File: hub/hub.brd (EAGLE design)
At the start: 28.2 x 25.4 mm, 5 parts

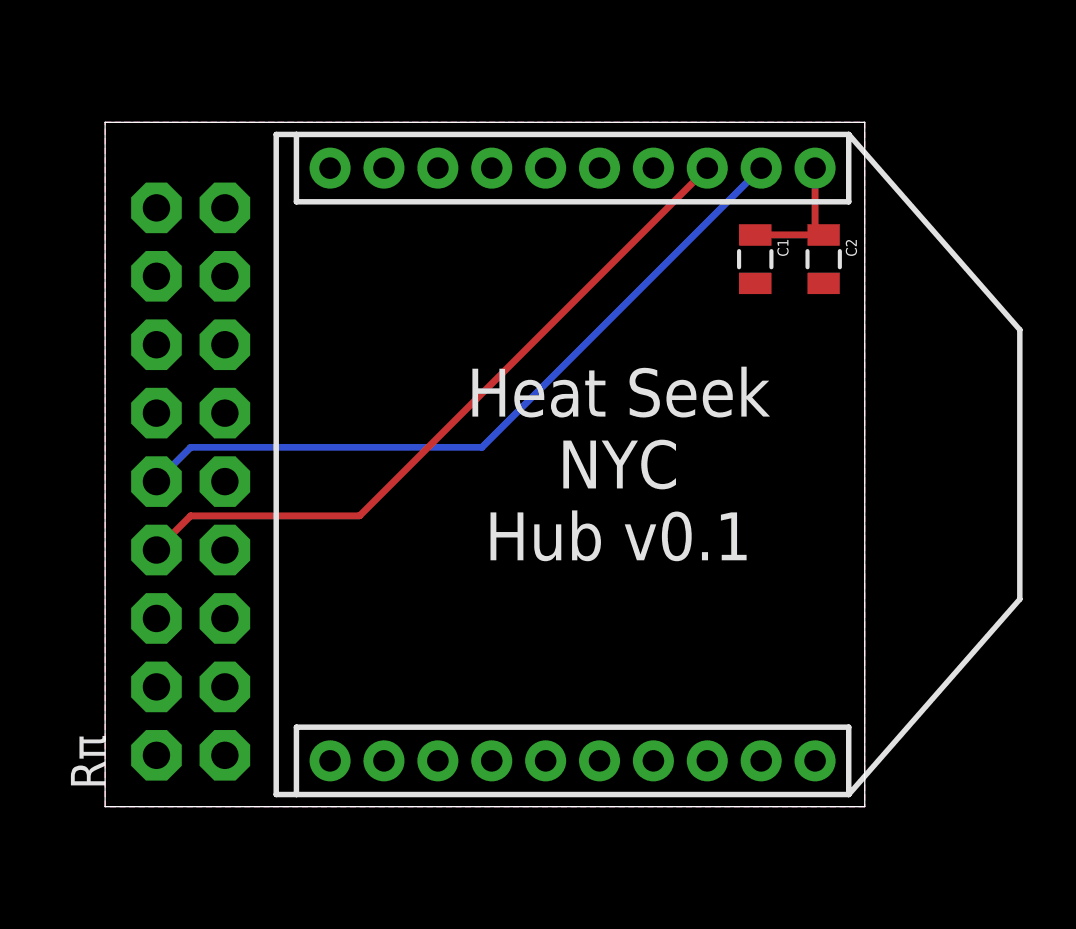
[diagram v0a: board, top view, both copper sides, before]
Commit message: smd-ver
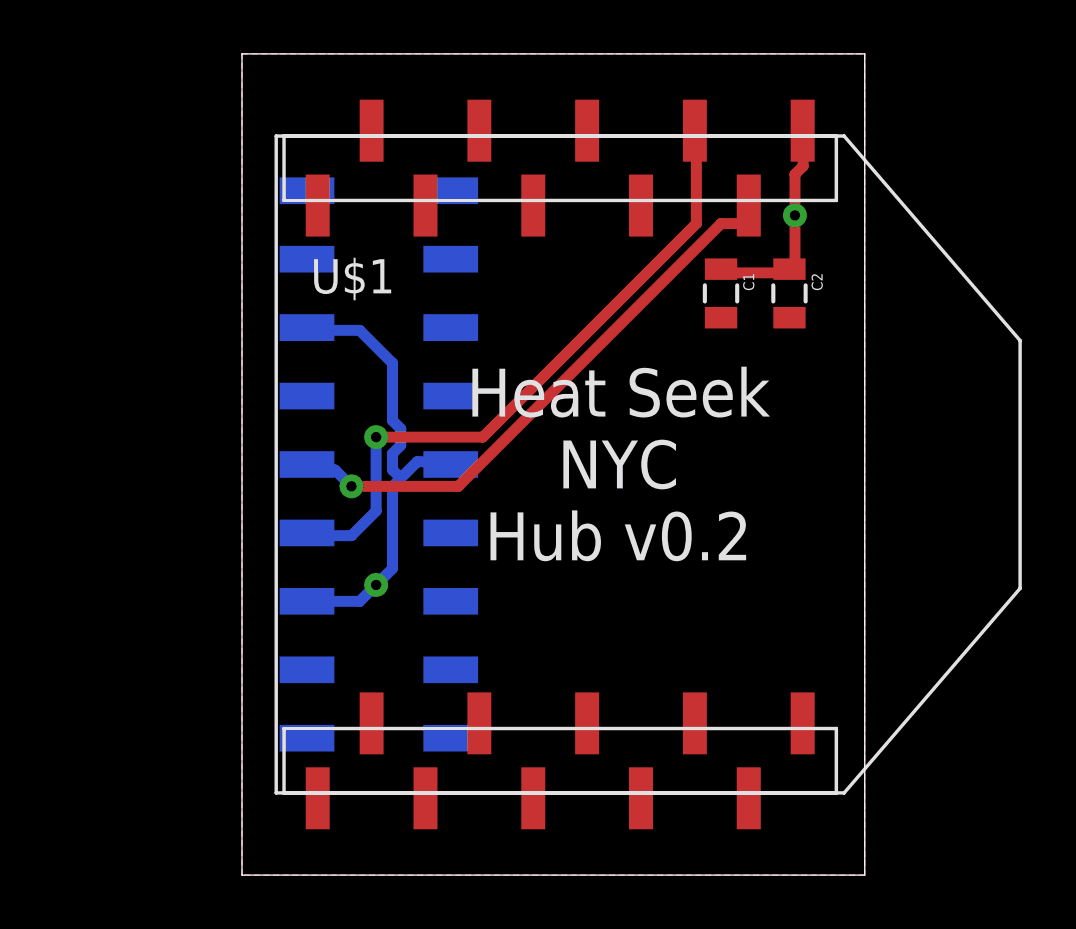
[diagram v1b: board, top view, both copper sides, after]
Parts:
- removed Rπ: M9X2, hrldcpr:2X9_NOSILK
- removed XB24: XBEE-1XBEE-1, hrldcpr:XBEE-1
- added 3.3VPI: S5718-NDSMD, heatseek_hub_smd_lib:CONN_HEADER_SMD_18
- added U$1: XBEESMD, heatseek_hub_smd_lib:CONN_HEADER_SMD_10X2
- moved C2 1.80 mm to (25.4, 19.1)
- moved C1 1.80 mm to (22.9, 19.1)
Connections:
- removed net VREF: XB24.14
- net 3.3V: now also 3.3VPI.1, 3.3VPI.17, U$1.1; no longer Rπ.1, Rπ.17, XB24.1
- net GND: now also 3.3VPI.14, 3.3VPI.6, 3.3VPI.9, U$1.10; no longer Rπ.14, Rπ.6, Rπ.9, XB24.10
- net N$1: now also 3.3VPI.10, U$1.2; no longer Rπ.10, XB24.2
- net N$2: now also 3.3VPI.8, U$1.3; no longer Rπ.8, XB24.3
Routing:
- net GND: track 0.00 -> 17.7 mm, vias 0 -> 1
- net N$1: track 27.3 -> 21.6 mm, vias 0 -> 1
- net 3.3V: track 5.34 -> 8.11 mm, vias 0 -> 1
- net N$2: track 26.3 -> 24.4 mm, vias 0 -> 1
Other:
- board size 28.2 x 25.4 mm -> 23.1 x 30.5 mm
- board text added: "Harold Cooper, Doyun Kim"
- board text added: "Heat Seek NYC Hub v0.2"
- board text removed: "Harold Cooper"
- board text removed: "Heat Seek NYC Hub v0.1"
